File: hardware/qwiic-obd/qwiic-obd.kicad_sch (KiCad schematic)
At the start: 8 parts, among them J101 I2C_STANDARD, J102 DB15_Female_HighDensity, J103 I2C_STANDARD

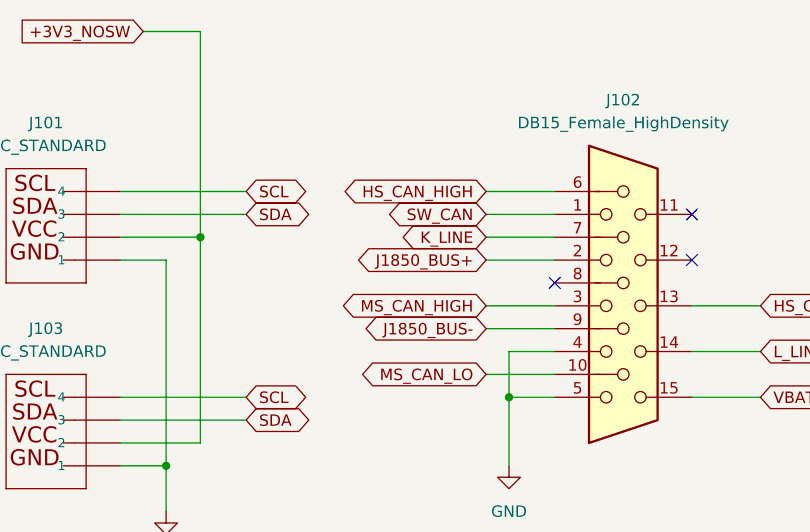
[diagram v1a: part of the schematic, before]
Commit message: OK, layout v1 complete
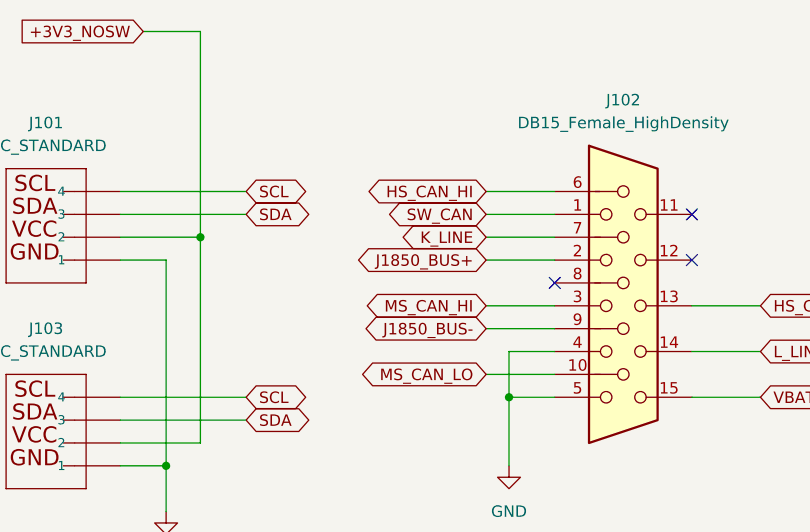
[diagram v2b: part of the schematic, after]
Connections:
- net HS_CAN_HIGH is gone; now on net HS_CAN_HI: J102.6
- net MS_CAN_HIGH is gone; now on net MS_CAN_HI: J102.3
